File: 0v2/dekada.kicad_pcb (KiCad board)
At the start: 2 copper layers, 52.3 x 34.1 mm, 43 parts, among them P1 CONN_02X10, P2 CONN_02X10, P3 CONN_02X10, P4 CONN_02X10, P5 CONN_01X02, P6 CONN_01X02, P7 CONN_01X02

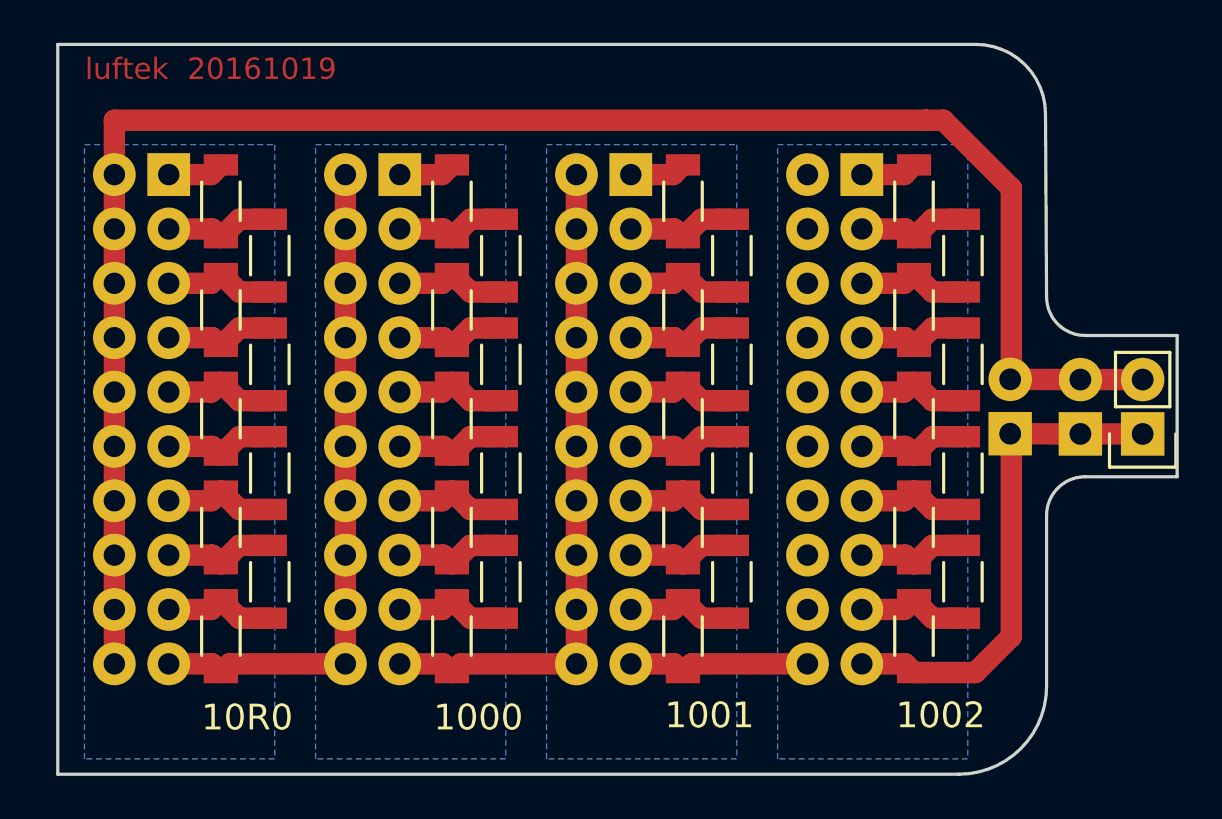
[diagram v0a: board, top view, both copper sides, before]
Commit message: Version 0v3
assembled, tested, working
no downsides or need for improvement found for now
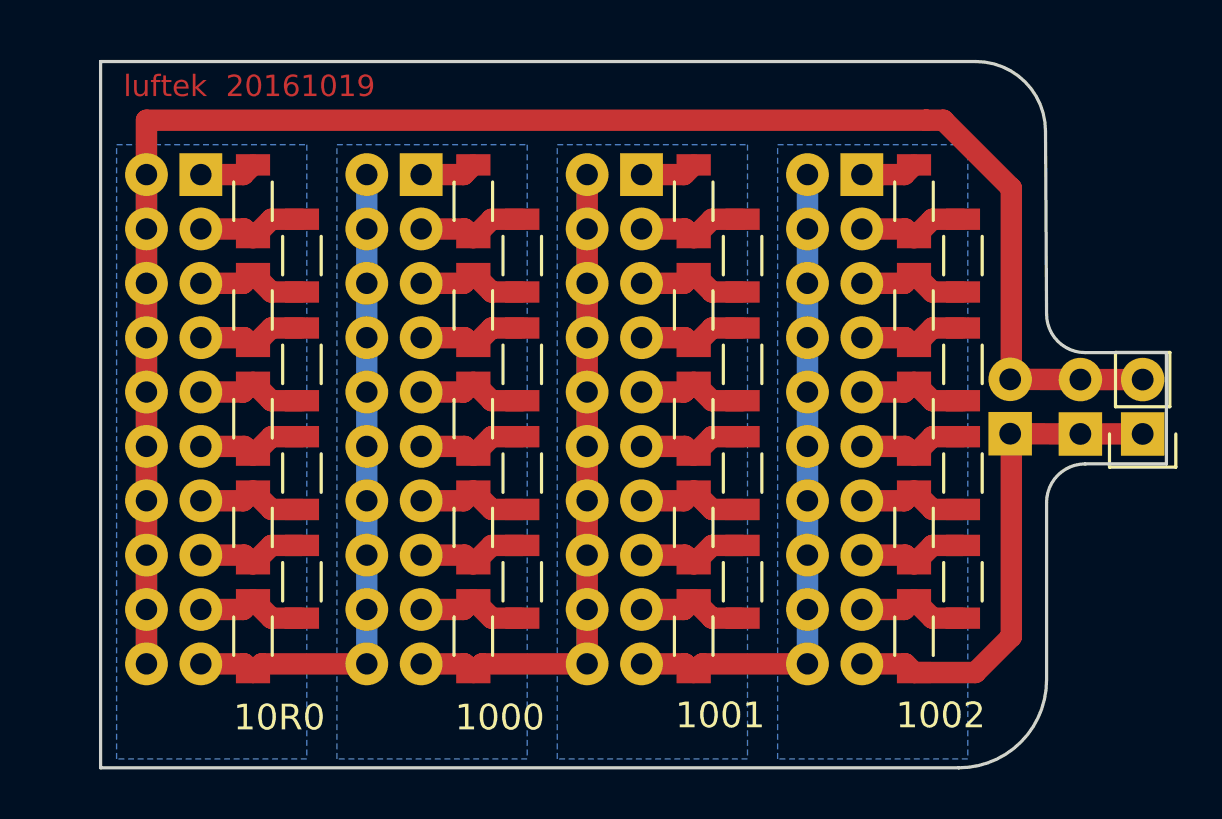
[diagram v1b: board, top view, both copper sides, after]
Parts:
- moved P1 1.50 mm to (88.4, 33.6)
- moved R1 1.50 mm to (90.8, 34.8)
- moved R2 1.50 mm to (93.1, 37.4)
- moved R3 1.50 mm to (90.8, 39.9)
- moved R4 1.50 mm to (93.1, 42.5)
- moved R5 1.50 mm to (90.8, 45.0)
- moved R6 1.50 mm to (93.1, 47.5)
- moved R7 1.50 mm to (90.8, 50.1)
- moved R8 1.50 mm to (93.1, 52.6)
- moved R9 1.50 mm to (90.8, 55.2)
- moved P2 1.00 mm to (98.7, 33.6)
- moved R11 1.00 mm to (101.1, 34.8)
- moved R12 1.00 mm to (103.4, 37.4)
- moved R13 1.00 mm to (101.1, 39.9)
- moved R14 1.00 mm to (103.4, 42.5)
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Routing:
- net Net-(P3-Pad19): track 8.59 -> 31.0 mm
- net Net-(P2-Pad19): track 31.5 -> 53.8 mm
- net Net-(P1-Pad10): track 84.0 -> 105.4 mm
- net Net-(P1-Pad19): track 31.5 -> 31.0 mm
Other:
- board size 52.3 x 34.1 mm -> 49.8 x 33 mm
